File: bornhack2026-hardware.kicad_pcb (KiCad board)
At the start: 4 copper layers, 67.5 x 90.1 mm, 147 parts, among them J1 USB device, J2 E-Paper, J9 Battery, Q1 JSM2301S, Q2 AP2302B, SW1 TS-1187A-B-A-B, SW2 SK-3296S-01-L1, SW3 SKRHABE010, SW6 TS3425PA 160GF 098, SW8 TS3425PA 160GF 098, U2 TPE4259-63, U3 SX1262IMLTRT, U4 XT4054K421MR-G, U5 ZD25WQ16CTIGT, U6 NRF52840-QIAA-R, U7 TPS63020DSJR, X1 S201632M10PF10PPM, X2 S201632M10PF10PPM, Y1 32.768KHz

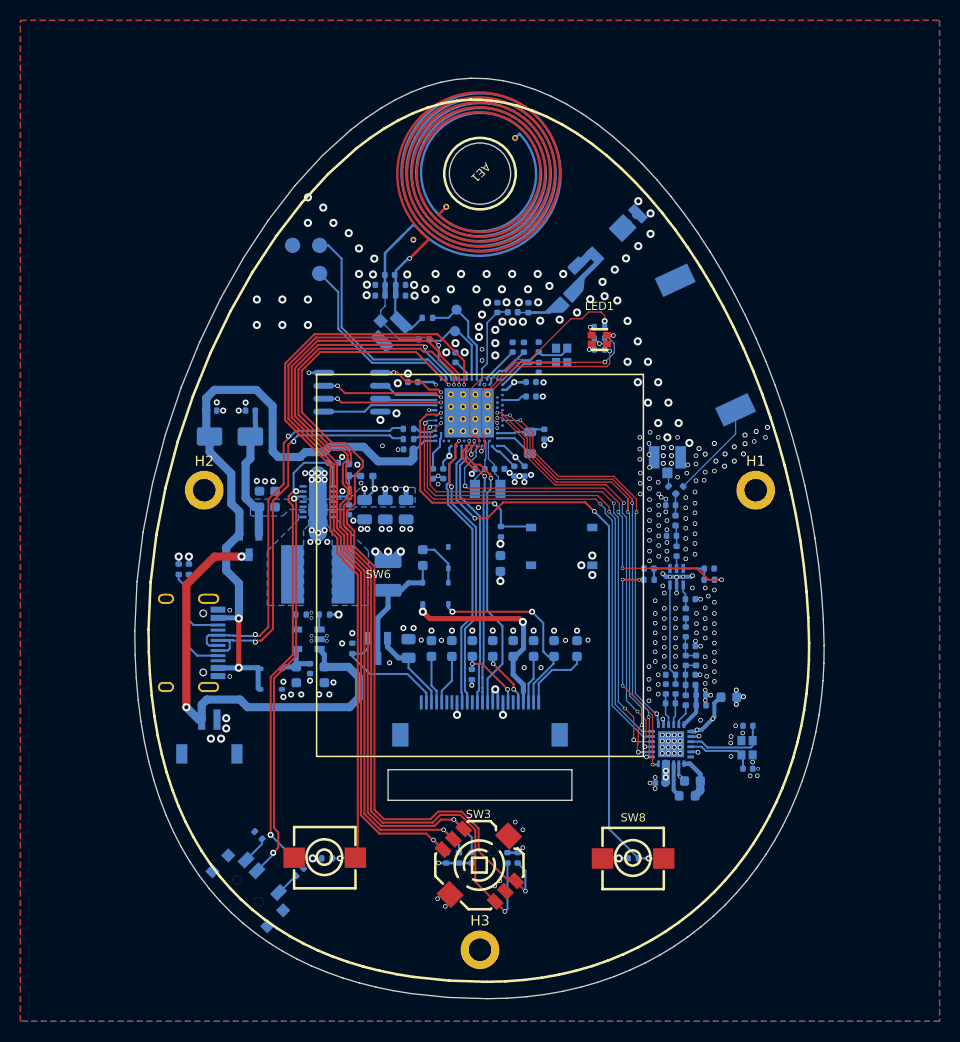
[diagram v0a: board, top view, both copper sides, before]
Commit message: Fixed DRC errors, added bunch of stitch through vias.
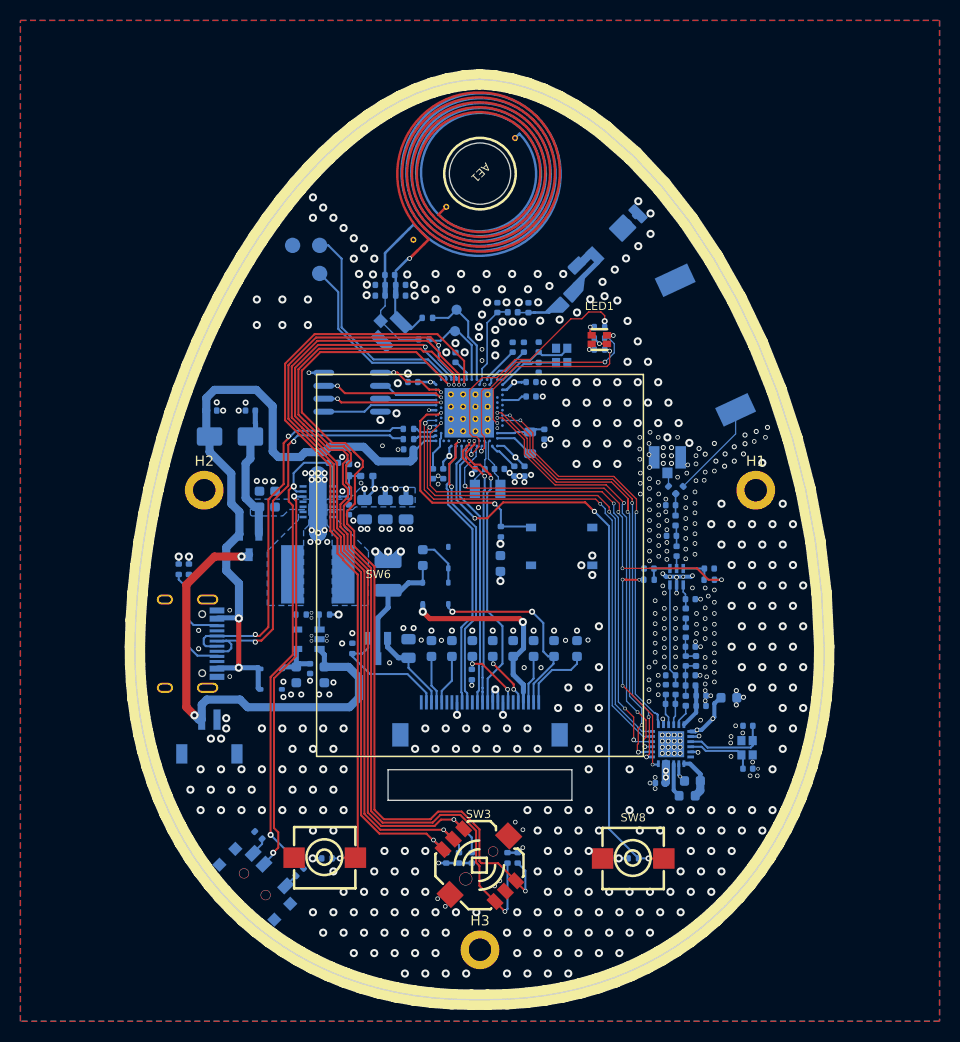
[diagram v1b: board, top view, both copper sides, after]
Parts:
- moved SW2 0.94 mm to (-21.7, 29.3)
- moved J1 0.13 mm to (-29.8, 6.03)
- moved C25 0.06 mm to (21.6, 12.1)
- moved C26 0.06 mm to (21.6, 11.1)
- moved C46 0.06 mm to (20.6, 9.13)
- moved C47 0.06 mm to (20.6, 6.33)
- moved C51 0.06 mm to (19.1, 10.5)
- moved C52 0.06 mm to (18.7, 9.13)
- moved C53 0.06 mm to (24.4, 11.3)
- moved L11 0.06 mm to (20.1, 11.6)
- moved L12 0.06 mm to (18.6, 11.9)
- moved L6 0.06 mm to (20.6, 10.1)
- moved L7 0.06 mm to (21.1, 7.73)
- moved C45 0.06 mm to (20.1, 7.73)
- moved C48 0.06 mm to (20.1, 4.93)
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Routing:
- net Net-(R14-Pad2): track 2.33 -> 1.43 mm
- net /USB_D+: track 39.5 -> 40.0 mm
- net /BTN_JOY_RIGHT: track 87.4 -> 88.0 mm
- net Net-(R16-Pad2): track 2.71 -> 2.18 mm
- net /P0.29_LORA_SPI_NSS: track 40.8 -> 40.5 mm, vias 3 -> 2
- net GND: vias 364 -> 598
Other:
- outline, holes or cut-outs redrawn
